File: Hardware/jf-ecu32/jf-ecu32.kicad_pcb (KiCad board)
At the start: 2 copper layers, 71.3 x 48.3 mm, 79 parts, among them J1 GAZ, J10 k, J11 RPM, J12 S.PORT, J13 PPM/PWM, J14 PUMP1, J15 PUMP1, J16 PPM/PWM, J17 PUMP2, J18 PUMP2, J19 UART0, J2 AUX, J3 PPM/PWM, J4 STARTER, J5 GLOW, J6 VANNE KEROSTART, J7 VANNE KERO, J8 BATTERY 2S/3S, J9 STARTER, Q1 AO3400A, Q2 QM6006D, Q3 AO3400A, Q4 QM6006D, Q5 QM6006D, Q6 QM6006D, Q7 AO3401A, U1 ESP32-WROOM-32D, U2 4050, U3 MAX31855KASA, U4 AMS1117-3.3, U5 4050, U6 AMS1117-5.0

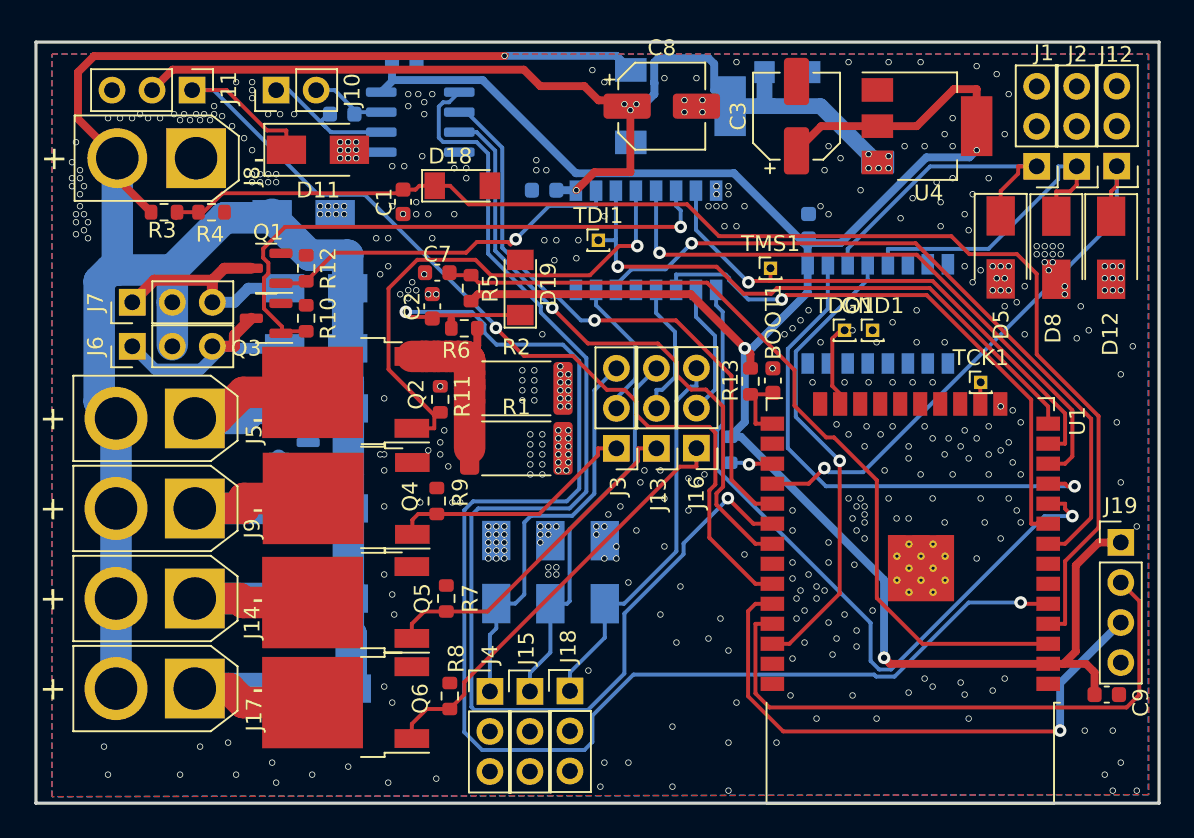
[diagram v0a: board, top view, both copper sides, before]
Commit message: PCB
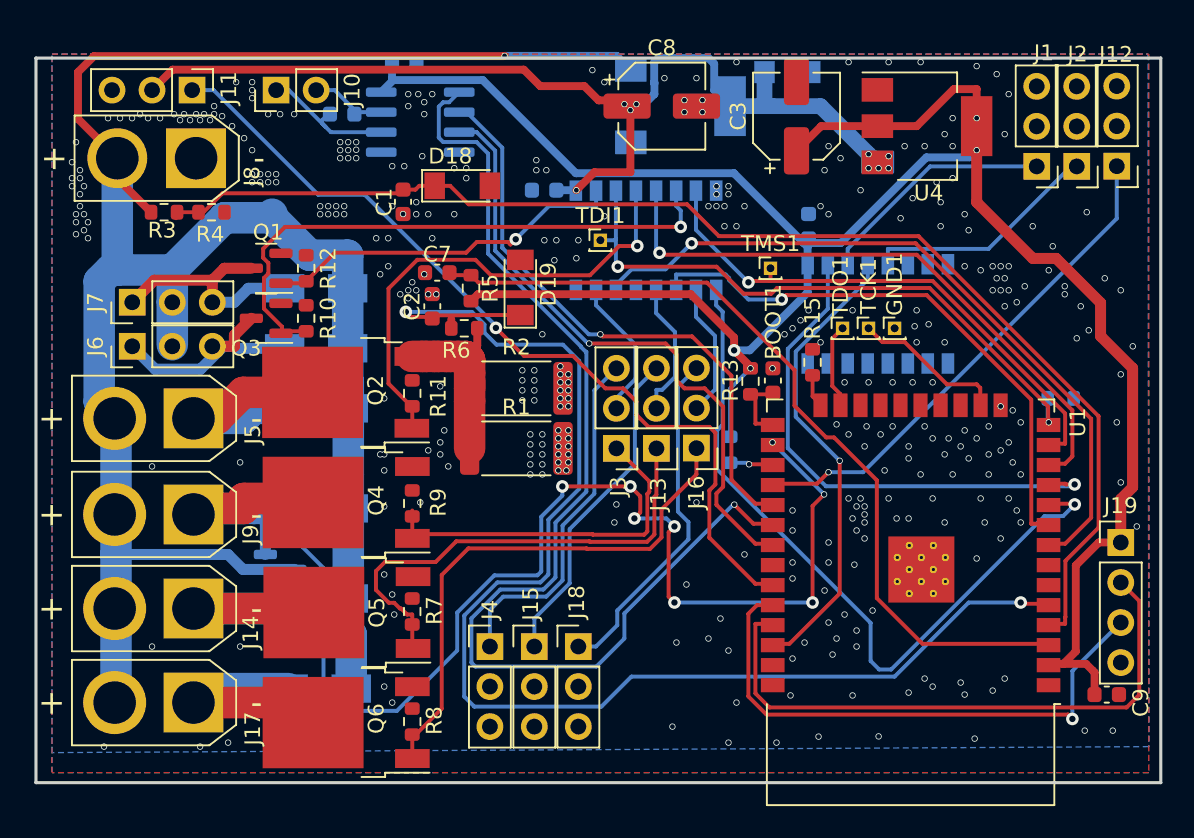
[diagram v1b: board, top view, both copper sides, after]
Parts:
- removed D11, D12, D14, D16, D4, D5, D6, D8: D_Schottky, Diode_SMD:D_SMA
- added R15: 10K, Resistor_SMD:R_0603_1608Metric, F.Cu at (62.0, 170.4)
- added R16: 10K, Resistor_SMD:R_0603_1608Metric, B.Cu at (77.7, 172.7)
- moved TCK1 7.90 mm to (65.5, 168.3)
- moved Q7 6.22 mm to (28.2, 182.6)
- moved R8 2.88 mm to (36.6, 193.2)
- moved J18 2.87 mm to (47.1, 188.5)
- moved J15 2.86 mm to (44.3, 188.5)
- moved J4 2.85 mm to (41.5, 188.5)
- moved R7 2.31 mm to (36.6, 186.2)
- moved R11 1.82 mm to (36.6, 172.4)
- moved R9 1.56 mm to (36.6, 179.4)
- moved GND1 1.40 mm to (67.2, 168.3)
- moved Q6 1.27 mm to (32.4, 193.3)
- moved J17 0.89 mm to (22.7, 192.0)
- moved J14 0.64 mm to (22.7, 186.1)
- moved Q5 0.64 mm to (32.4, 186.3)
- moved J9 0.39 mm to (22.7, 180.1)
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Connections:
- Q7 pad 1: unconnected-(Q7-Pad1) -> BRAKE
- U1 pad 24: unconnected-(U1-Pad24) -> Net-(U1-Pad24)
- U1 pad 26: unconnected-(U1-Pad26) -> BRAKE
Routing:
- net BRAKE: track 0.00 -> 71.5 mm, vias 0 -> 8
- net +BATT: track 133.8 -> 143.1 mm
- net Net-(J13-Pad1): track 21.5 -> 30.5 mm
- net RPM: track 63.1 -> 54.8 mm
- net TCK: track 1.37 -> 9.49 mm
- net CLK: track 79.4 -> 71.6 mm
- net Net-(J3-Pad1): track 16.0 -> 22.7 mm
- net Net-(J16-Pad1): track 27.4 -> 34.1 mm
- net GLOW_CURRENT: track 93.2 -> 86.6 mm
- net PPM_GAZ_5V: track 19.9 -> 15.1 mm
- net AUX_5V: track 19.8 -> 15.1 mm
- net 3.3V: track 141.4 -> 145.7 mm, vias 3 -> 4
- net Net-(J13-Pad3): track 24.5 -> 20.9 mm
- net TX2: track 35.7 -> 32.1 mm
- net Net-(J3-Pad3): track 26.1 -> 22.6 mm
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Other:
- board size 71.3 x 48.3 mm -> 71.4 x 46 mm

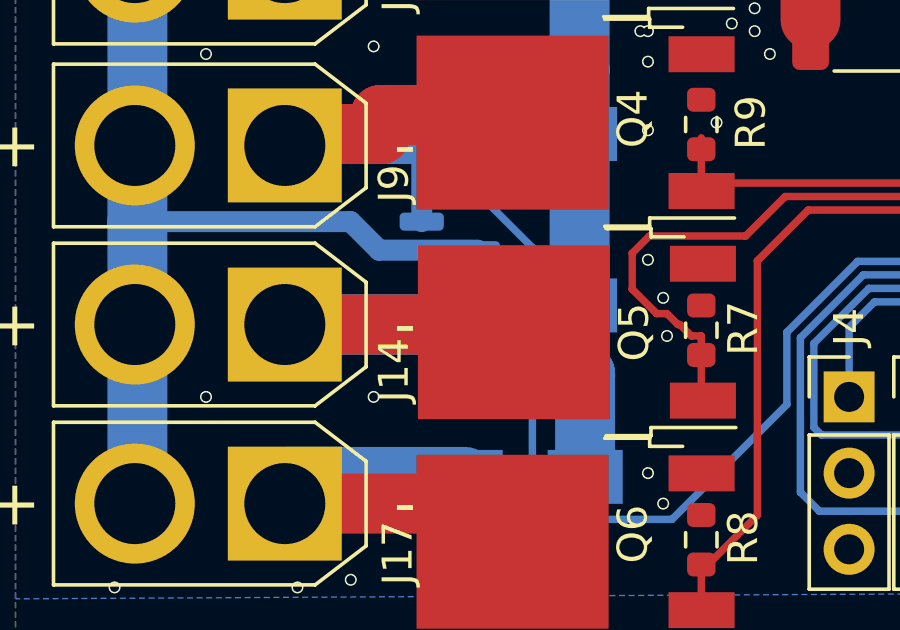
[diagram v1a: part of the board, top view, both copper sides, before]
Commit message: SCH + PCB
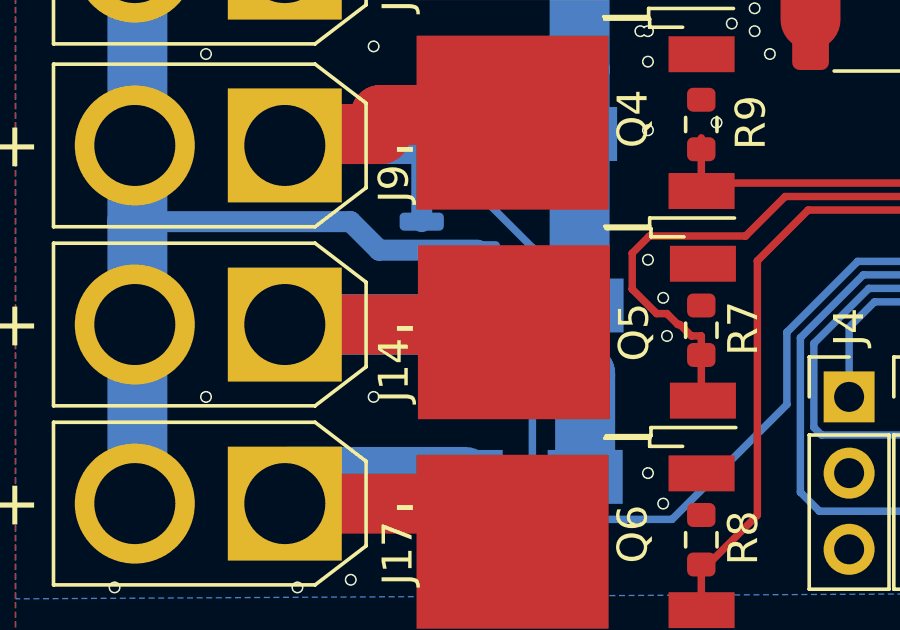
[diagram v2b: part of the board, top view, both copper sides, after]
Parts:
- moved D13 0.21 mm to (30.7, 185.4)
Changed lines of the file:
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@@
   )
   (footprint "Diode_SMD:D_SMA" (layer "B.Cu")
-    (at 30.52 185.42 180)
+    (at 30.734 185.42 180)
     (descr "Diode SMA (DO-214AC)")
     (tags "Diode SMA (DO-214AC)")
@@
   (segment (start 22.78 185.42) (end 23.415 186.055) (width 2) (layer "F.Cu") (net 37))
   (segment (start 23.415 186.055) (end 29.87 186.055) (width 2) (layer "F.Cu") (net 37))
-  (segment (start 27.885 186.055) (end 23.415 186.055) (width 2) (layer "B.Cu") (net 37))
-  (segment (start 28.52 185.42) (end 27.885 186.055) (width 2) (layer "B.Cu") (net 37))
+  (segment (start 28.099 186.055) (end 23.415 186.055) (width 2) (layer "B.Cu") (net 37))
+  (segment (start 28.734 185.42) (end 28.099 186.055) (width 2) (layer "B.Cu") (net 37))
   (segment (start 23.415 186.055) (end 22.78 185.42) (width 2) (layer "B.Cu") (net 37))
   (segment (start 42.418 151.003) (end 16.383 151.003) (width 0.5) (layer "F.Cu") (net 38))
